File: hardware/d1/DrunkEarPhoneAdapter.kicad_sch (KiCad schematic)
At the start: 0 parts

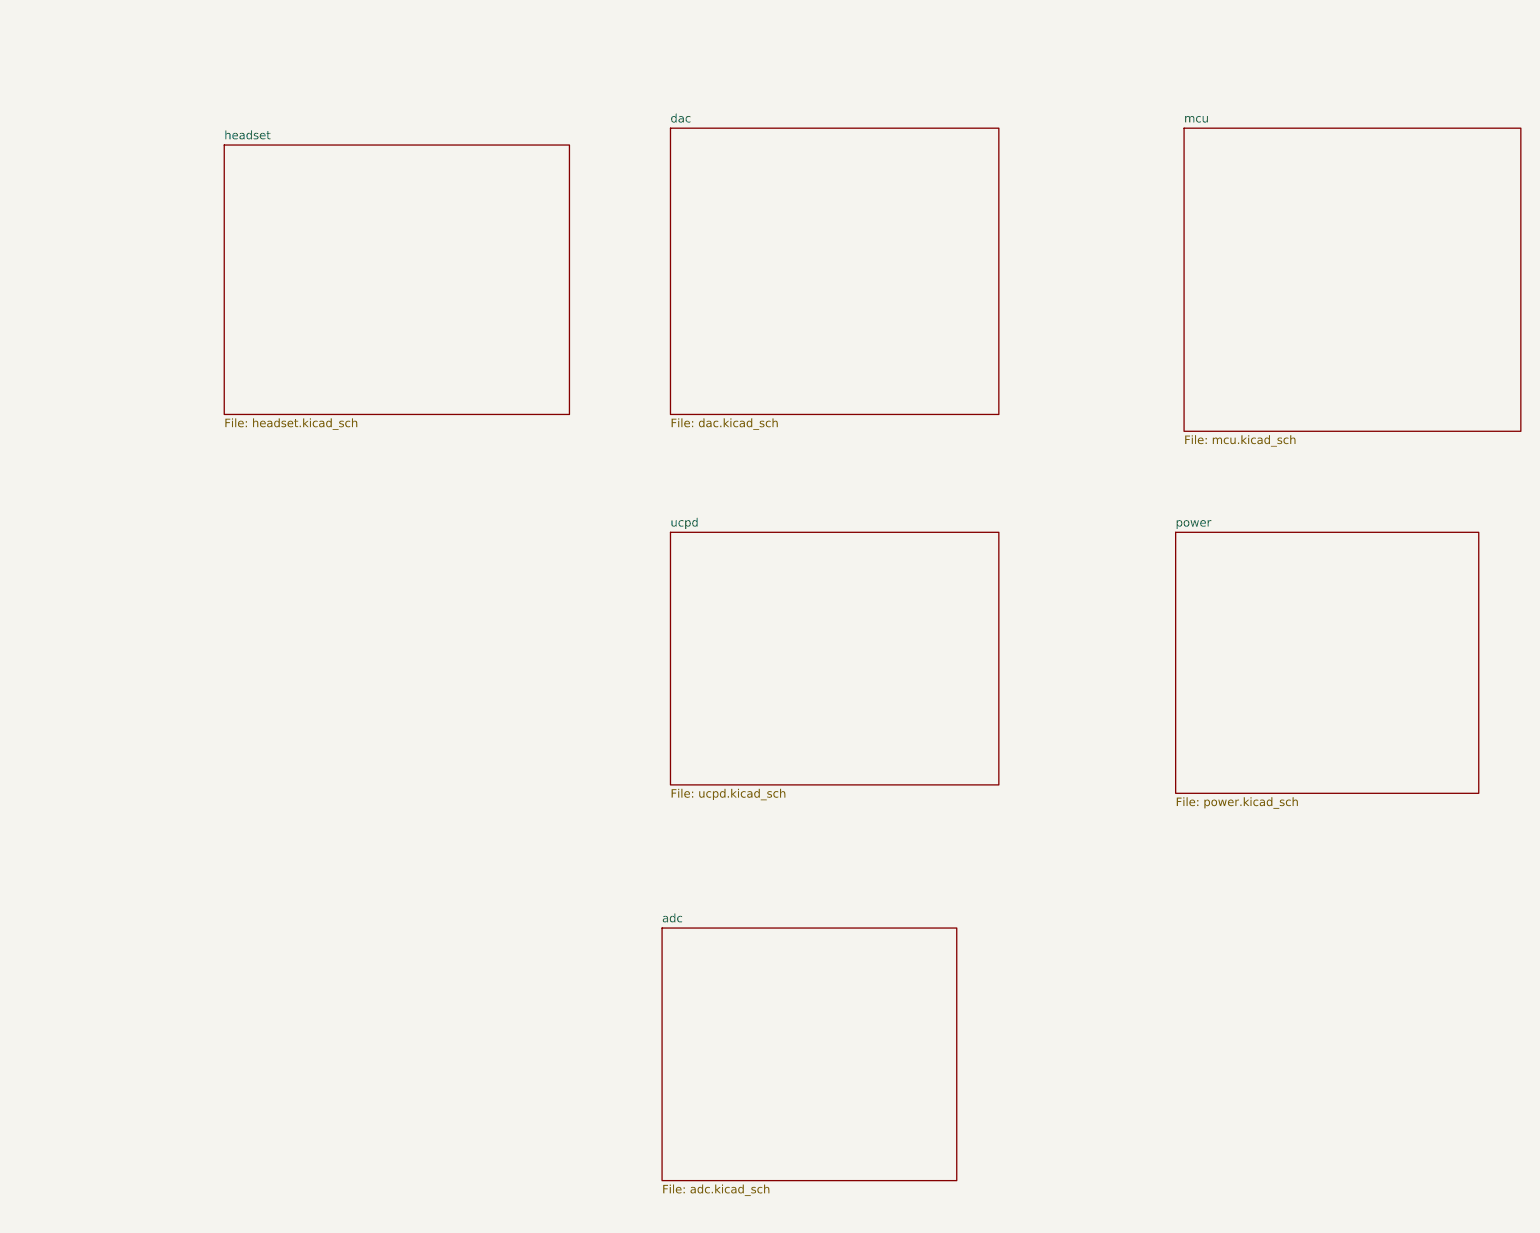
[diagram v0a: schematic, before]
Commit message: Pre-finalize sch
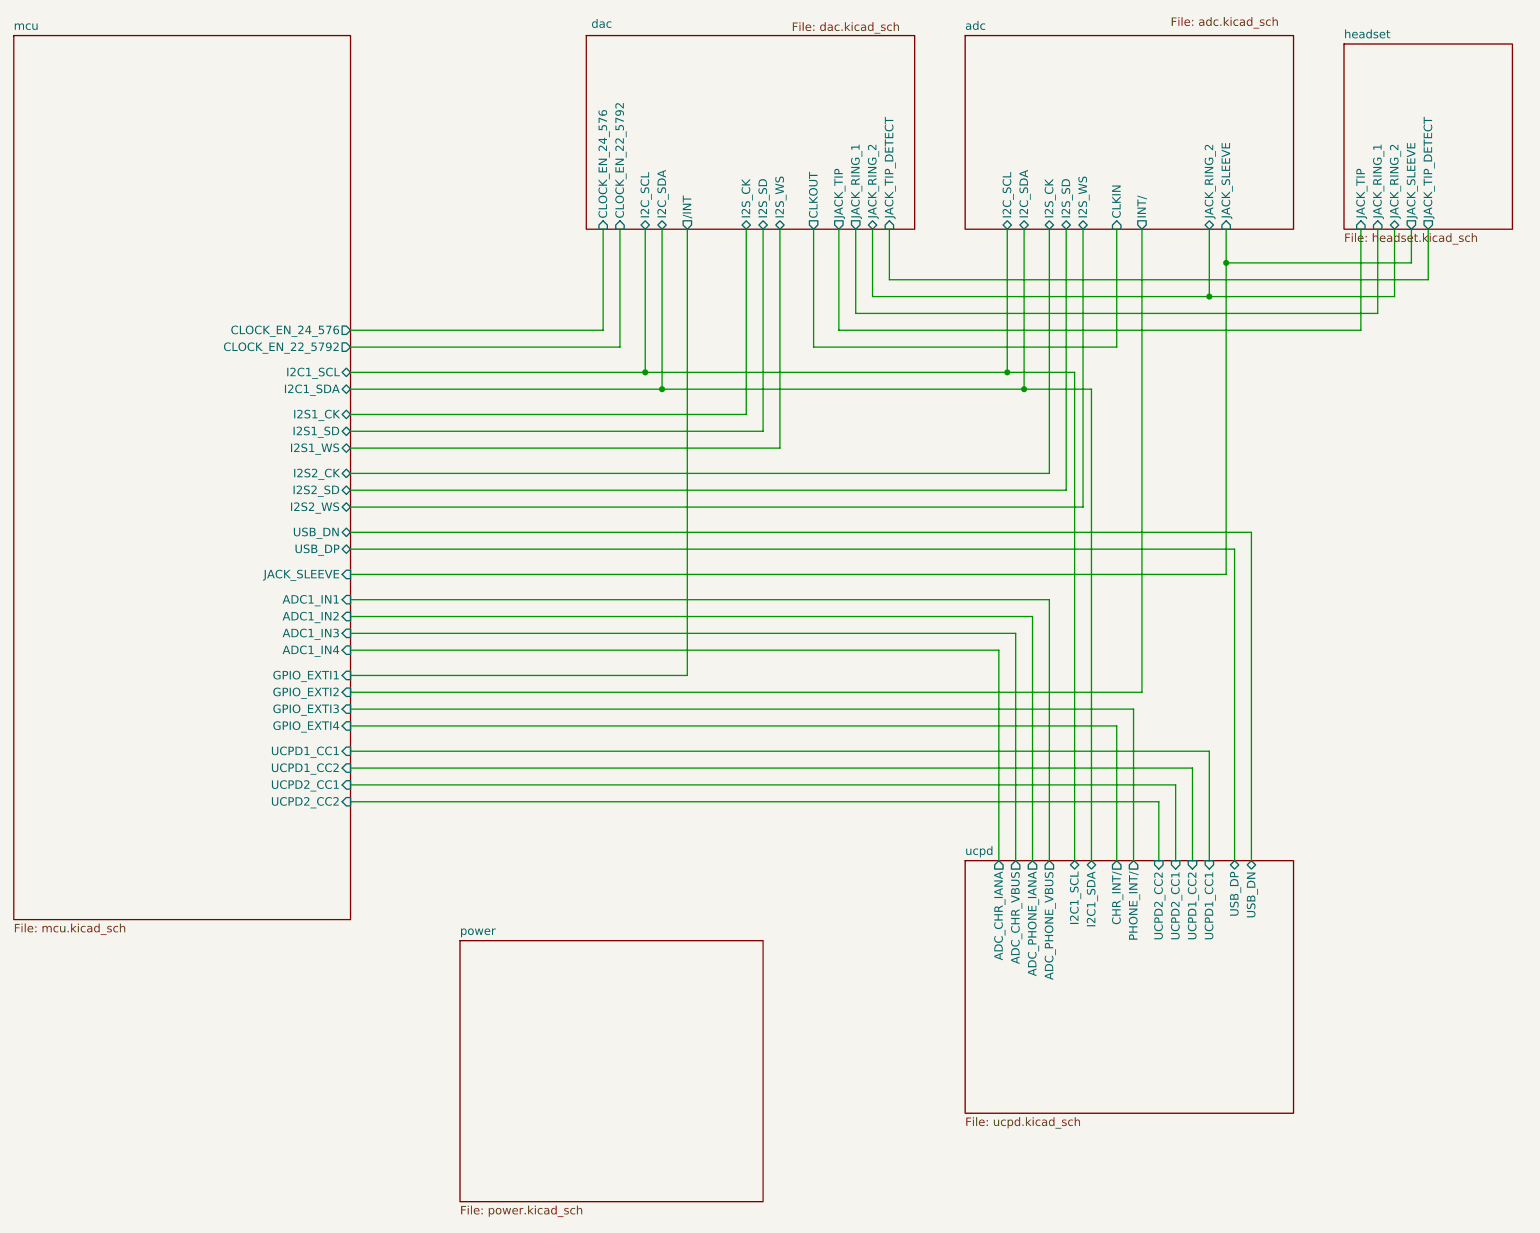
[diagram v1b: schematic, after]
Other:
- sheet adc ports: added CLKIN, I2C_SCL, I2C_SDA, I2S_CK, I2S_SD, I2S_WS, INT/, JACK_RING_2, JACK_SLEEVE; removed none
- sheet dac ports: added CLKOUT, CLOCK_EN_22_5792, CLOCK_EN_24_576, I2C_SCL, I2C_SDA, I2S_CK, I2S_SD, I2S_WS, JACK_RING_1, JACK_RING_2, JACK_TIP, JACK_TIP_DETECT, /INT; removed none
- sheet headset ports: added JACK_RING_1, JACK_RING_2, JACK_SLEEVE, JACK_TIP, JACK_TIP_DETECT; removed none
- sheet mcu ports: added ADC1_IN1, ADC1_IN2, ADC1_IN3, ADC1_IN4, CLOCK_EN_22_5792, CLOCK_EN_24_576, GPIO_EXTI1, GPIO_EXTI2, GPIO_EXTI3, GPIO_EXTI4, I2C1_SCL, I2C1_SDA, I2S1_CK, I2S1_SD, I2S1_WS, I2S2_CK, I2S2_SD, I2S2_WS, JACK_SLEEVE, UCPD1_CC1, UCPD1_CC2, UCPD2_CC1, UCPD2_CC2, USB_DN, USB_DP; removed none
- sheet ucpd ports: added ADC_CHR_IANA, ADC_CHR_VBUS, ADC_PHONE_IANA, ADC_PHONE_VBUS, CHR_INT/, I2C1_SCL, I2C1_SDA, PHONE_INT/, UCPD1_CC1, UCPD1_CC2, UCPD2_CC1, UCPD2_CC2, USB_DN, USB_DP; removed none
